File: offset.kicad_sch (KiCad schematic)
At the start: 52 parts

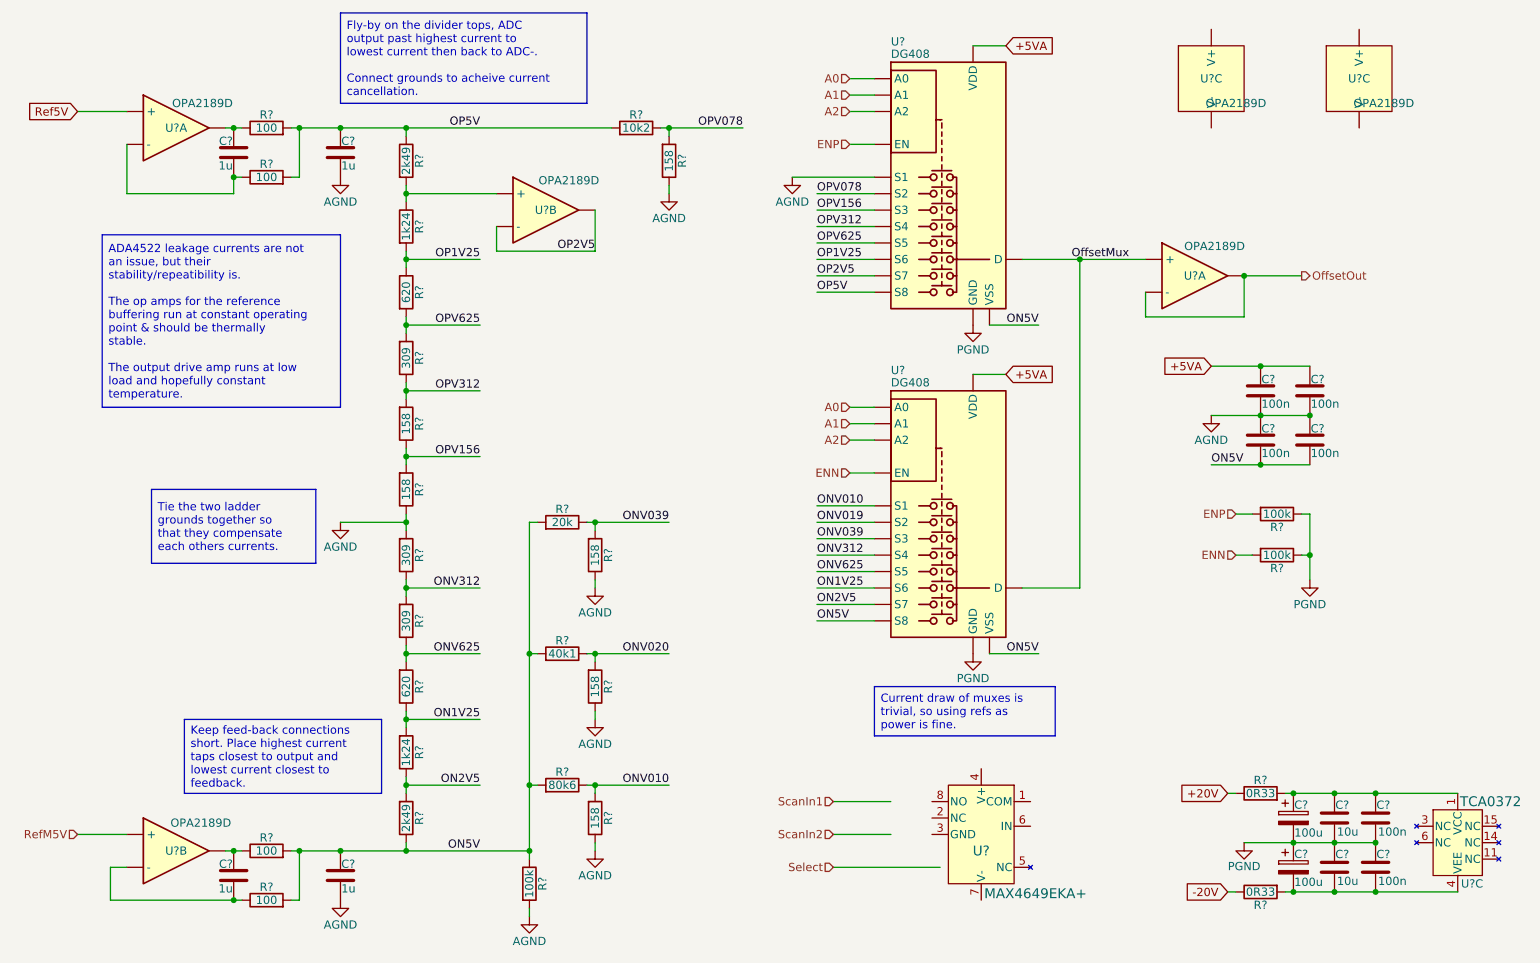
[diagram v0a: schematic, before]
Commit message: More work in progres
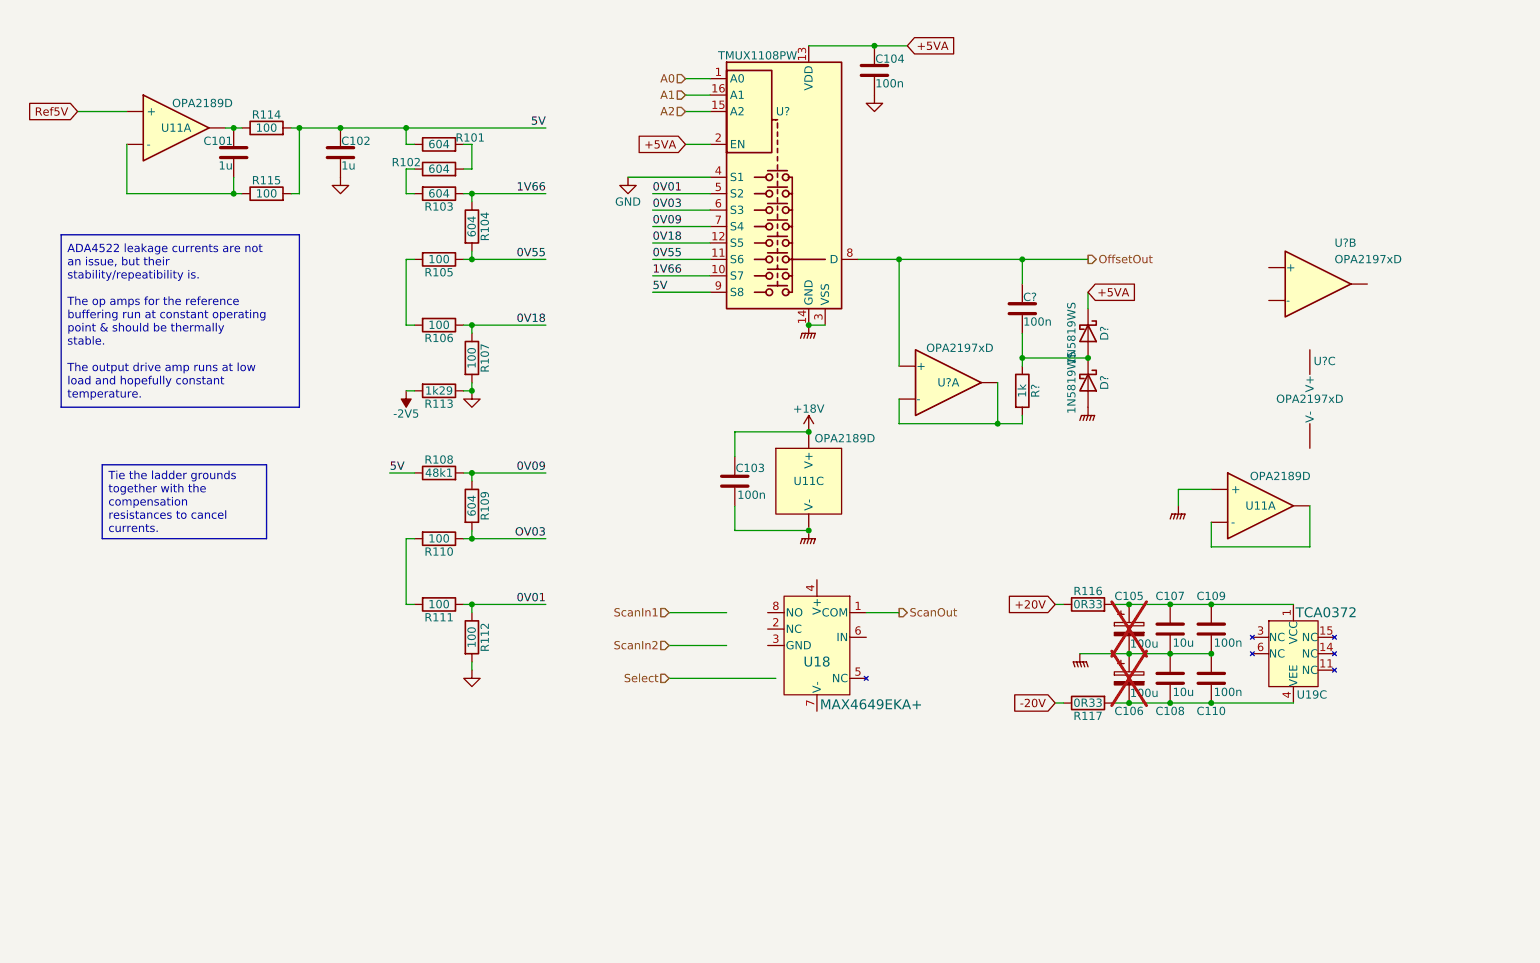
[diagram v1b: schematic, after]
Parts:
- removed C? (x3): 100n, symbol Device:C
- removed C? (x2): 1u, symbol Device:C
- removed R? (x3): 100k, symbol Device:R
- removed R? (x6): 158, symbol Device:R
- removed R? (x3): 309, symbol Device:R
- removed R?: 10k2, symbol Device:R
- removed R? (x2): 620, symbol Device:R
- removed R?: 80k6, symbol Device:R
- removed R?: 40k1, symbol Device:R
- removed R? (x2): 2k49, symbol Device:R
- removed R? (x2): 100, symbol Device:R
- removed R?: 20k, symbol Device:R
- removed R?: 1k24, symbol Device:R
- removed U? (x3): OPA2189D, Package_SO:SOIC-8_3.9x4.9mm_P1.27mm, symbol Parts:OPA2189D
- removed U? (x2): DG408, Package_SO:TSSOP-16_4.4x5mm_P0.65mm, symbol Analog_Switch:ADG1408YRUZ
- added C103, C?: 100n, symbol Device:C
- added D? (x2): 1N5819WS, Diode_SMD:D_SOD-323, symbol Diode:1N5819WS
- added R101, R102, R103, R109: 604, Resistor_SMD:R_0603_1608Metric, symbol Device:R
- added R105, R106, R107, R110, R111, R112: 100, Resistor_SMD:R_0603_1608Metric, symbol Device:R
- added R108: 48k1, Resistor_SMD:R_0603_1608Metric, symbol Device:R
- added R113: 1k29, Resistor_SMD:R_0603_1608Metric, symbol Device:R
- added R?: 1k, Resistor_SMD:R_0402_1005Metric, symbol Device:R
- added U?: TMUX1108PW, Package_SO:TSSOP-16_4.4x5mm_P0.65mm, symbol Analog_Switch:TMUX1108PW
- added U? (x3): OPA2197xD, Package_SO:SOIC-8_3.9x4.9mm_P1.27mm, symbol Amplifier_Operational:OPA2197xD
- C105, C106: renamed from C?; now not fitted
- R104: renamed from R?; value 1k24 -> 604; footprint (none) -> Resistor_SMD:R_0603_1608Metric
- R114, R115: renamed from R?; footprint (none) -> Resistor_SMD:R_0402_1005Metric
- R116, R117: renamed from R?; footprint (none) -> Resistor_SMD:R_0805_2012Metric
- gave numbers to parts that had none: 10
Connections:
- net OffsetMux is gone; now on net GNDPWR: U11.3 (+)
- net PGND is gone; now on net GNDPWR: C105.2, C106.1, C107.2, C108.1, C109.2, C110.1
- net +5VA: now also D?.1 (K), U?.13 (VDD), U?.2 (EN)
- net A0: now also U?.1 (A0)
- net A1: now also U?.16 (A1)
- net A2: now also U?.15 (A2)
- net OffsetOut: now also C?.1, U?.3 (+), U?.8 (D); no longer U11.1, U11.2 (-)
- net 1V66: now reaches R104.1
- net 1V66: now also R103.1, U?.10 (S7)
- net GNDPWR: now reaches U11.4 (V-)
- net GNDPWR: now also C103.2, D?.2 (A), U?.14 (GND), U?.3 (VSS)
- net +18V: now reaches U11.8 (V+)
- net +18V: now also C103.1
- net ScanOut: now reaches U18.1 (COM)
- net AGND renamed GND
- net GND: now also R107.2, R112.2, R113.1, U?.4 (S1)
- net OP1V25 renamed 0V55
- net 0V55: now also R105.1, U?.11 (S6)
- net OP5V renamed 5V
- net 5V: now also R101.1, R108.1, U?.9 (S8)
- new net: R101.2, R102.2
- new net: C?.2, D?.1 (K), D?.2 (A), R?.1
- new net: R105.2, R106.2
- new net: R102.1, R103.2
- new net: R?.2, U?.1, U?.2 (-)
- new net: R110.2, R111.2
- new net: U11.1, U11.2 (-)
- new net -2V5: R113.2
- new net 0V01: R111.1, R112.1, U?.5 (S2)
- new net 0V03: U?.6 (S3)
- new net 0V09: R108.2, R109.1, U?.7 (S4)
- new net 0V18: R106.1, R107.1, U?.12 (S5)
- new net OV03: R109.2, R110.1
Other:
- moved on the sheet: C104, C107, C108, C109, C110, R104, R115, R116, R117, U11A, U11C, U18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
